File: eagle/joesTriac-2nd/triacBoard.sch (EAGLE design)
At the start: 12 parts, among them X1 1751316, X2 1751248

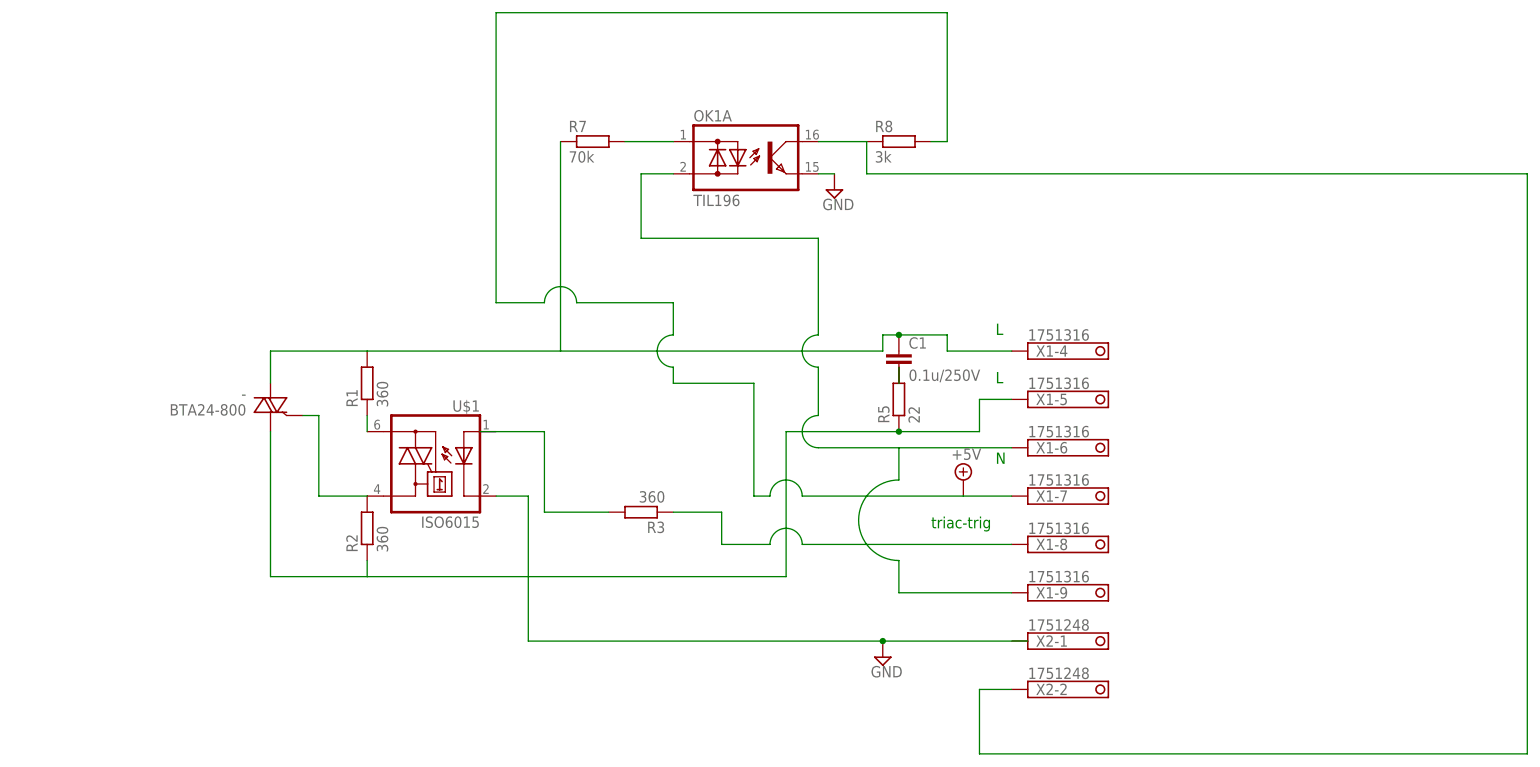
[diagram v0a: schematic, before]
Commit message: reg save, runs as never before :-), EAGLE CHANGES
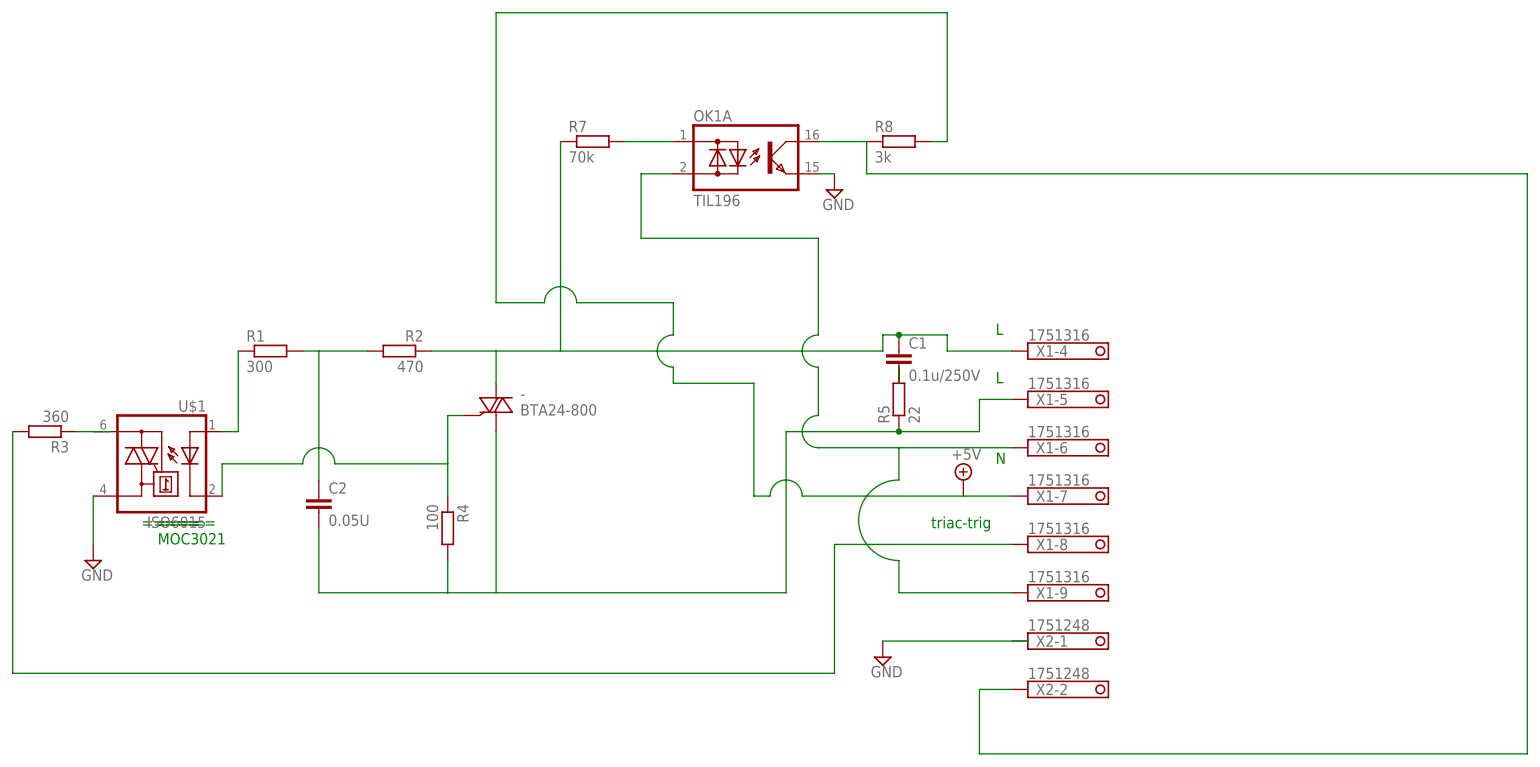
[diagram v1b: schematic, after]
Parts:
- added C2: 0.05U, resistor:C-EU025-040X050
- added R4: 100, resistor:R-EU_0207/15
- R1: value 360 -> 300
- R2: value 360 -> 470
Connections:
- removed net N$12: R3.1, X1-8.K
- new net N$10: -.A2, C1.1, R2.1, R7.1, X1-4.K
- new net N$2: C2.2, R4.2, R5.1, X1-5.K
- new net N$3: R3.1
- new net N$9: -.A1
- net GND: now also U$1.A1; no longer U$1.C
- net N$11: now also R4.1, U$1.C; no longer R3.2
- net N$4: now also -.G; no longer -.A2, C1.1, R1.2, R7.1, X1-4.K
- net N$5: now also C2.1, R1.2, R2.2; no longer -.A1, R2.1, R5.1, X1-5.K
- net N$6: now also R3.2, X1-8.K; no longer R1.1, U$1.A2
- net N$7: now also R1.1, U$1.A; no longer -.G, R2.2, U$1.A1
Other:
- note added: "====="
- note added: "MOC3021"
- moved on the sheet: -, R1, R2, R3, U$1

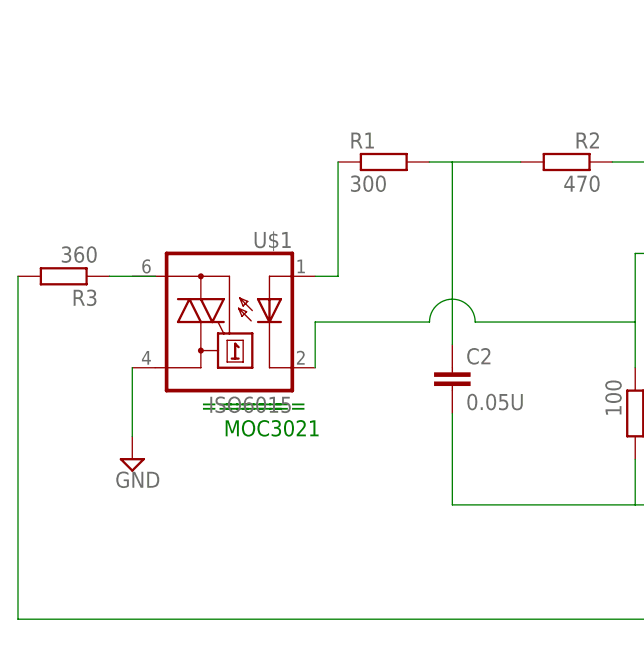
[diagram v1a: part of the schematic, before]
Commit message: reg save, minor changes
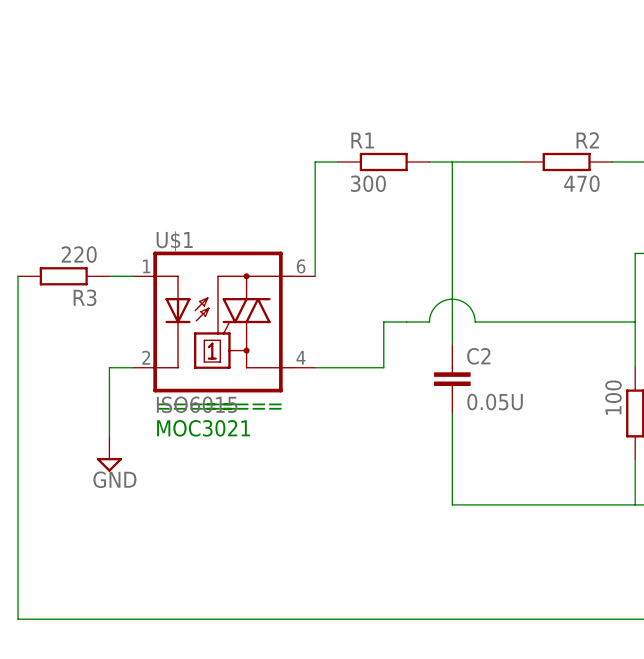
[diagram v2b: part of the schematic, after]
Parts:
- R3: value 360 -> 220
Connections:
- removed net N$11: R4.1, U$1.C
- removed net N$3: R3.1
- new net N$12: R4.1, U$1.A1
- new net N$13: R3.1, U$1.A
- net GND: now also U$1.C; no longer U$1.A1
- net N$7: now also U$1.A2; no longer U$1.A
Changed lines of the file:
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@@
 <part name="R7" library="resistor" deviceset="R-EU_" device="0207/15" value="70k"/>
 <part name="R8" library="resistor" deviceset="R-EU_" device="0207/15" value="3k"/>
-<part name="R3" library="resistor" deviceset="R-EU_" device="0207/15" value="360"/>
+<part name="R3" library="resistor" deviceset="R-EU_" device="0207/15" value="220"/>
 <part name="SUPPLY4" library="supply2" deviceset="GND" device=""/>
 <part name="SUPPLY1" library="supply2" deviceset="GND" device=""/>
@@
 <text x="45.72" y="71.12" size="1.778" layer="91">N</text>
 <text x="35.56" y="60.96" size="1.778" layer="91">triac-trig</text>
-<text x="-86.36" y="58.42" size="1.778" layer="91">MOC3021</text>
-<text x="-86.36" y="60.96" size="1.778" layer="91">=====</text>
+<text x="-93.98" y="58.42" size="1.778" layer="91">MOC3021</text>
+<text x="-93.98" y="60.96" size="1.778" layer="91">=====</text>
 <text x="-88.9" y="60.96" size="1.778" layer="91">=====</text>
 </plain>
@@
 <instance part="X2" gate="-1" x="50.8" y="43.18"/>
 <instance part="X2" gate="-2" x="50.8" y="35.56"/>
-<instance part="U$1" gate="G$1" x="-86.36" y="71.12" rot="MR0"/>
+<instance part="U$1" gate="G$1" x="-86.36" y="71.12"/>
 <instance part="R1" gate="G$1" x="-68.58" y="88.9"/>
 <instance part="R2" gate="G$1" x="-48.26" y="88.9" rot="MR0"/>
@@
 <instance part="R3" gate="G$1" x="-104.14" y="76.2" rot="R180"/>
 <instance part="SUPPLY4" gate="GND" x="20.32" y="114.3"/>
-<instance part="SUPPLY1" gate="GND" x="-96.52" y="55.88"/>
+<instance part="SUPPLY1" gate="GND" x="-99.06" y="55.88"/>
 <instance part="C2" gate="G$1" x="-60.96" y="66.04"/>
 <instance part="R4" gate="G$1" x="-40.64" y="60.96" rot="R270"/>
@@
 </segment>
 <segment>
-<pinref part="U$1" gate="G$1" pin="A1"/>
-<wire x1="-96.52" y1="66.04" x2="-96.52" y2="58.42" width="0.1524" layer="91"/>
+<pinref part="U$1" gate="G$1" pin="C"/>
+<wire x1="-96.52" y1="66.04" x2="-99.06" y2="66.04" width="0.1524" layer="91"/>
 <pinref part="SUPPLY1" gate="GND" pin="GND"/>
+<wire x1="-99.06" y1="66.04" x2="-99.06" y2="58.42" width="0.1524" layer="91"/>
 </segment>
 </net>
@@
 </segment>
 </net>
-<net name="N$3" class="0">
-<segment>
-<pinref part="R3" gate="G$1" pin="1"/>
-<wire x1="-99.06" y1="76.2" x2="-93.98" y2="76.2" width="0.1524" layer="91"/>
-</segment>
-</net>
 <net name="N$6" class="0">
 <segment>
@@
 <net name="N$7" class="0">
 <segment>
-<pinref part="U$1" gate="G$1" pin="A"/>
+<pinref part="U$1" gate="G$1" pin="A2"/>
+<wire x1="-76.2" y1="76.2" x2="-76.2" y2="88.9" width="0.1524" layer="91"/>
 <pinref part="R1" gate="G$1" pin="1"/>
-<wire x1="-76.2" y1="76.2" x2="-73.66" y2="76.2" width="0.1524" layer="91"/>
-<wire x1="-73.66" y1="76.2" x2="-73.66" y2="88.9" width="0.1524" layer="91"/>
+<wire x1="-76.2" y1="88.9" x2="-73.66" y2="88.9" width="0.1524" layer="91"/>
 </segment>
 </net>
@@
 </segment>
 </net>
-<net name="N$11" class="0">
-<segment>
-<pinref part="U$1" gate="G$1" pin="C"/>
-<wire x1="-76.2" y1="66.04" x2="-76.2" y2="71.12" width="0.1524" layer="91"/>
-<wire x1="-76.2" y1="71.12" x2="-63.5" y2="71.12" width="0.1524" layer="91"/>
+<net name="N$12" class="0">
+<segment>
+<pinref part="U$1" gate="G$1" pin="A1"/>
+<wire x1="-76.2" y1="66.04" x2="-68.58" y2="66.04" width="0.1524" layer="91"/>
+<wire x1="-68.58" y1="66.04" x2="-68.58" y2="71.12" width="0.1524" layer="91"/>
 <wire x1="-63.5" y1="71.12" x2="-58.42" y2="71.12" width="0.1524" layer="91" curve="-180"/>
 <wire x1="-58.42" y1="71.12" x2="-40.64" y2="71.12" width="0.1524" layer="91"/>
 <pinref part="R4" gate="G$1" pin="1"/>
 <wire x1="-40.64" y1="71.12" x2="-40.64" y2="66.04" width="0.1524" layer="91"/>
-</segment>
-</net>
+<wire x1="-68.58" y1="71.12" x2="-66.04" y2="71.12" width="0.1524" layer="91"/>
+<wire x1="-63.5" y1="71.12" x2="-66.04" y2="71.12" width="0.1524" layer="91"/>
+</segment>
+</net>
+<net name="N$13" class="0">
+<segment>
+<pinref part="U$1" gate="G$1" pin="A"/>
+<pinref part="R3" gate="G$1" pin="1"/>
+<wire x1="-99.06" y1="76.2" x2="-96.52" y2="76.2" width="0.1524" layer="91"/>
+</segment>
+</net>
